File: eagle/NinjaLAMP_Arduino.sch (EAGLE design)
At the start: 13 parts

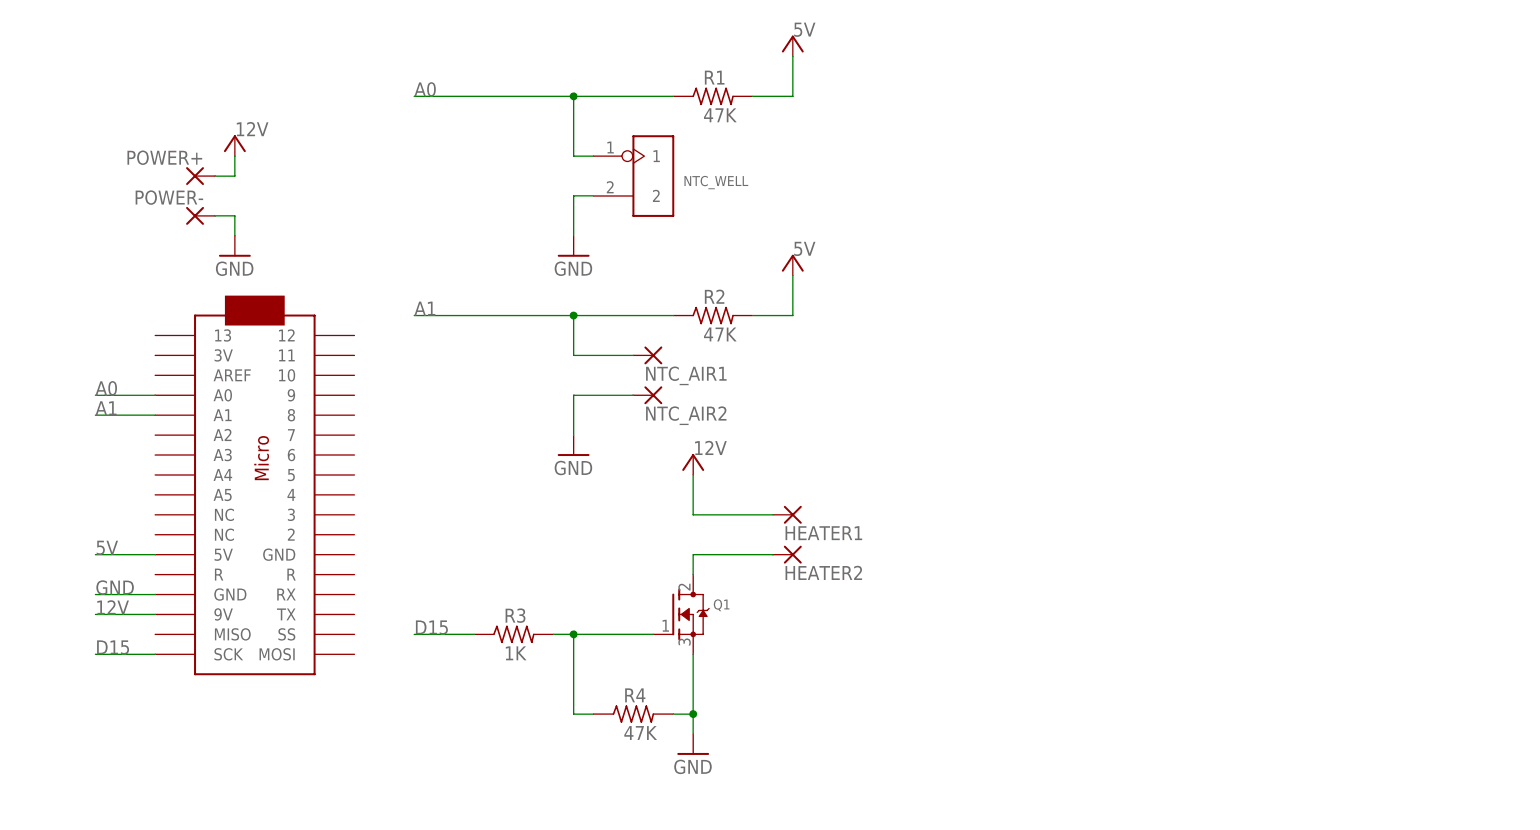
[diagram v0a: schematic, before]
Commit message: t5.5 lasercut design finished
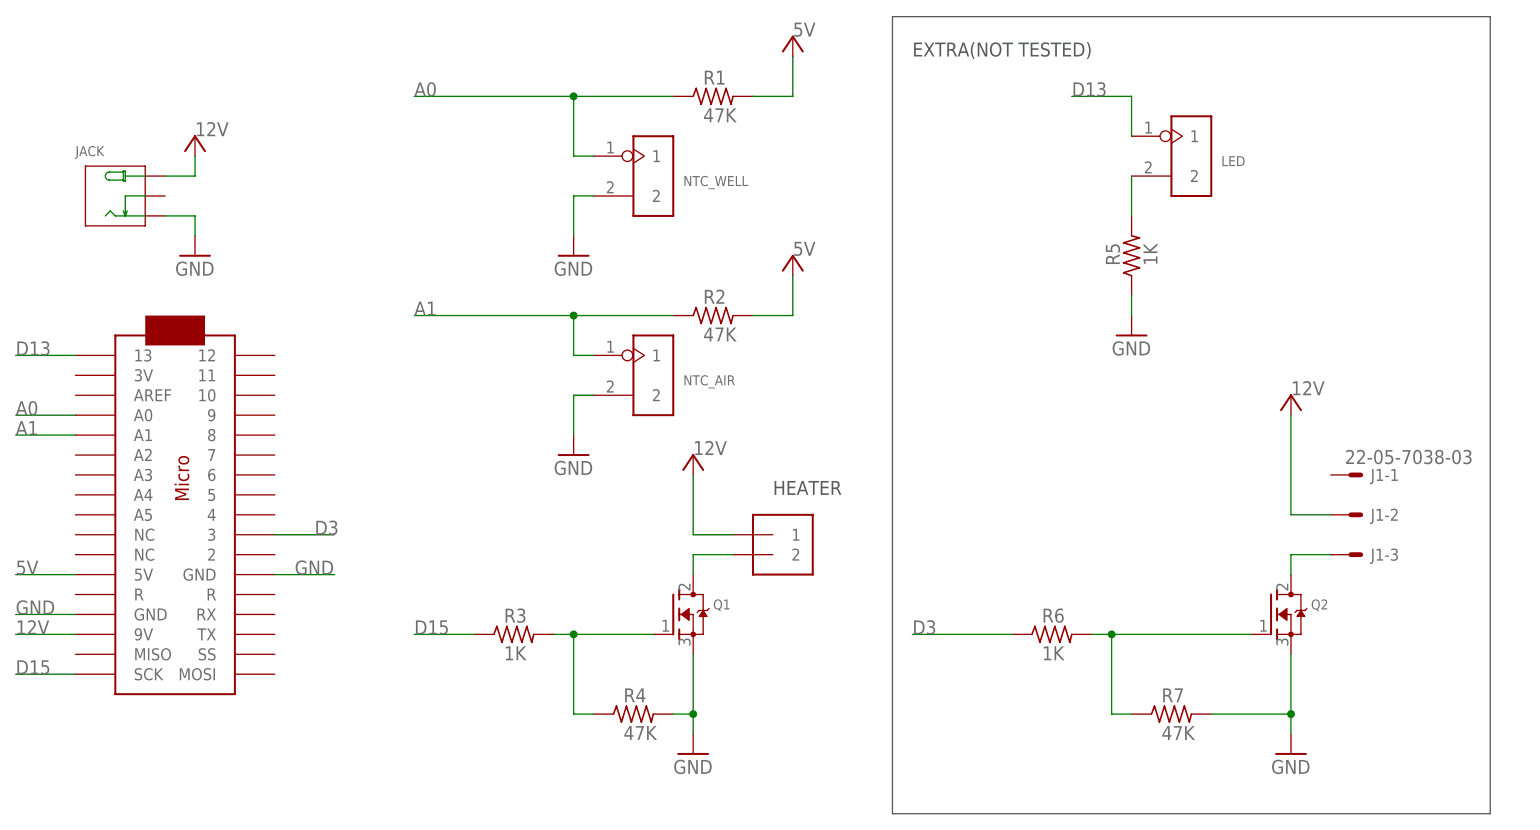
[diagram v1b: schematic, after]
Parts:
- removed HEATER1, HEATER2, NTC_AIR1, NTC_AIR2, POWER+, POWER-: (no value), wirepad:1,6/0,8
- removed U$1: ARDUINOMICRO, adafruit:ARDUINOMICRO
- added HEATER: 1X2-3.5MM, adafruit:1X2-3.5MM
- added J1: 22-05-7038-03, con-molex:22-05-7038-03
- added JACK: DC-005, OPL_Connector:CONN-POWER-JACK-2.1MM(DC-005)
- added LED, NTC_AIR: 2p-2.54, OPL_Connector:DIP-BLACK-MALE-HEADER-VERT(2P-2.54)
- added Q2: (no value), adafruit:MOSFET-NGDS_TO220V
- added R5, R6: 1K, resistor:R-US_0204/7
- added R7: 47K, resistor:R-US_0204/7
- added U$2: ARDUINOMICRO, adafruit:ARDUINOMICRO
- R1, R2, R3, R4: device resistor:R-US_0207/10 -> resistor:R-US_0204/7
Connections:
- new net D13: LED.1, U$2.13
- new net D3: R6.1, U$2.3
- new net N$2: LED.2, R5.2
- new net N$3: Q2.G, R6.2, R7.1
- new net N$6: J1-3.S, Q2.D
- net 12V: now also HEATER.1, J1-2.S, JACK.+, U$2.9V; no longer HEATER1.P, POWER+.P, U$1.9V
- net 5V: now also U$2.5V; no longer U$1.5V
- net A0: now also U$2.A0; no longer U$1.A0
- net A1: now also NTC_AIR.1, U$2.A1; no longer NTC_AIR1.P, U$1.A1
- net D15: now also U$2.SCK; no longer U$1.SCK
- net DRAIN: now also HEATER.2; no longer HEATER2.P
- net GND: now also JACK.-, NTC_AIR.2, Q2.S, R5.1, R7.2, U$2.GND, U$2.GND@1; no longer NTC_AIR2.P, POWER-.P, U$1.GND
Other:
- note added: "EXTRA(NOT TESTED)"
- note added: "HEATER"
